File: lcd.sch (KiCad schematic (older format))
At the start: 13 parts, among them J10 FH26W-33S-0.3SHW, J7 AFA07-S10FCC-00, U8 AP3019A

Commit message: cleaned up libs
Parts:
- U8: symbol otter:AP3019A -> OtterCastAmp-rescue:AP3019A-otter
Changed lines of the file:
@@
 LEDK
 $Comp
-L otter:AP3019A U8
+L OtterCastAmp-rescue:AP3019A-otter U8
 U 1 1 60C69466
 P 3550 2350

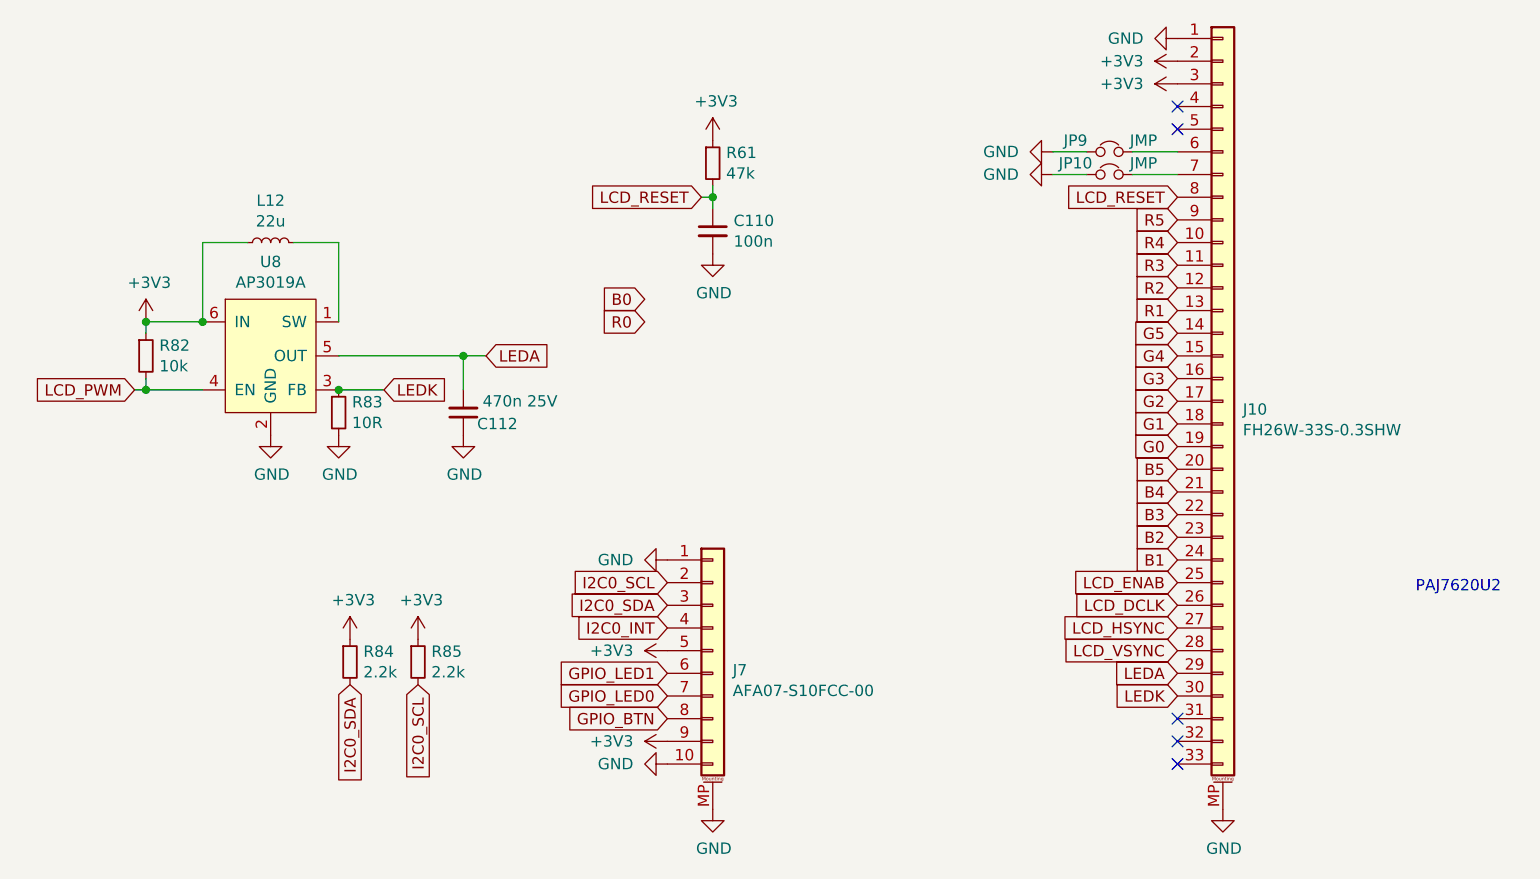
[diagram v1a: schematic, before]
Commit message: V1.2 production release
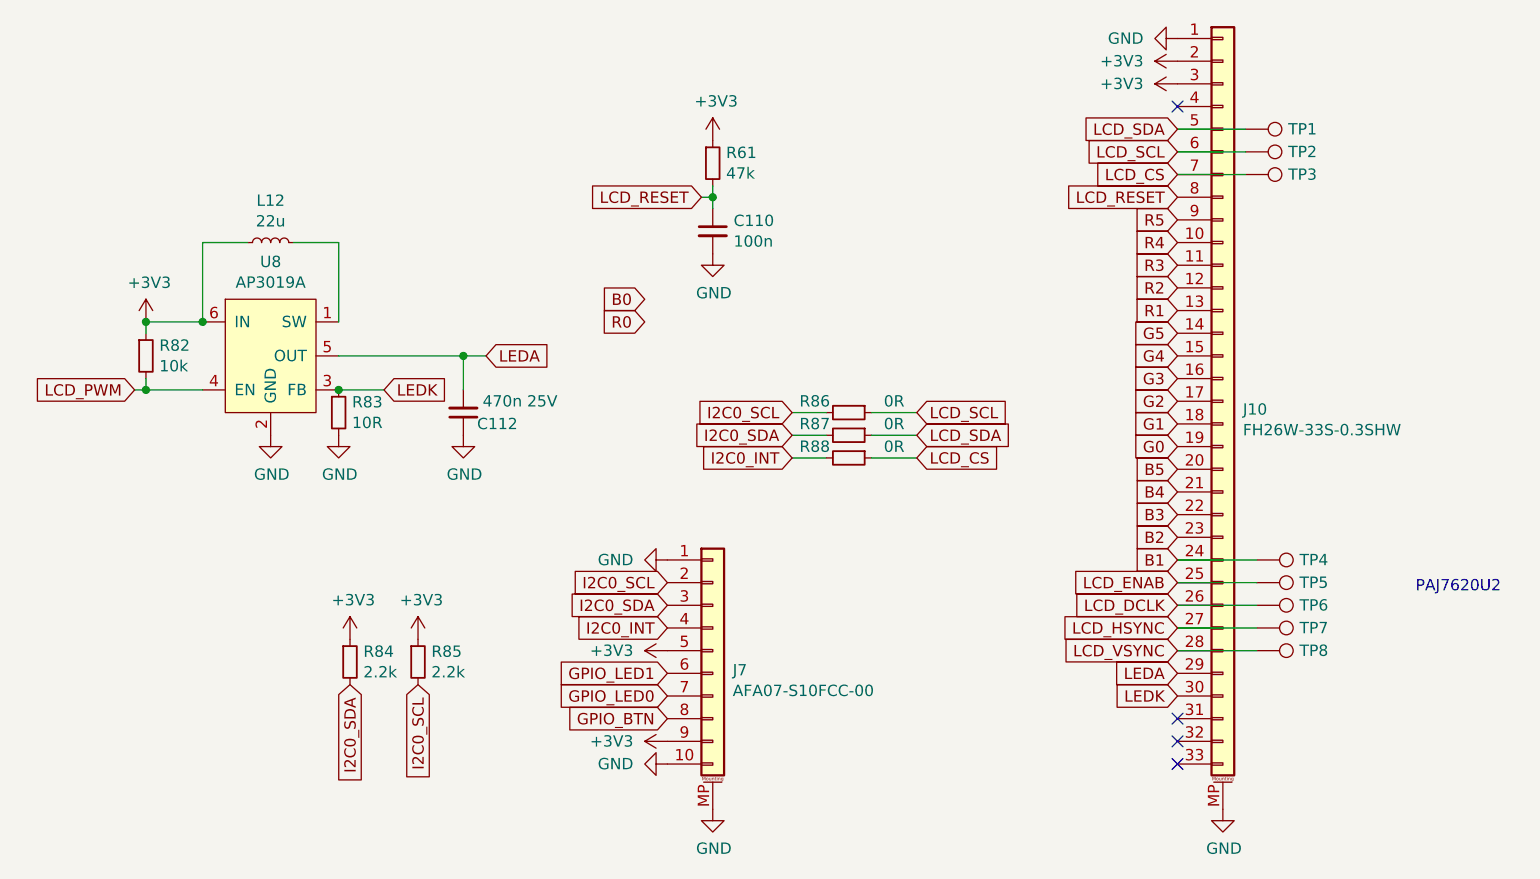
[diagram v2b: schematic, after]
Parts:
- removed JP10, JP9: JMP, Jumper:SolderJumper-2_P1.3mm_Bridged_Pad1.0x1.5mm, symbol Device:Jumper_NC_Small
- added R86, R87, R88: 0R, otter:R_0402, symbol Device:R_Small
- added TP1, TP2, TP3, TP4, TP5, TP6, TP7, TP8: TestPoint, TestPoint:TestPoint_Pad_1.0x1.0mm, symbol Connector:TestPoint
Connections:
- net B1: now also TP4.1
- net I2C0_INT: now also R88.2
- net I2C0_SCL: now also R86.2
- net I2C0_SDA: now also R87.2
- net LCD_DCLK: now also TP6.1
- net LCD_ENAB: now also TP5.1
- net LCD_HSYNC: now also TP7.1
- net LCD_VSYNC: now also TP8.1
- net LCD_SCL: now reaches J10.6 (Pin_6)
- net LCD_SCL: now also R86.1, TP2.1
- net LCD_CS: now reaches J10.7 (Pin_7)
- net LCD_CS: now also R88.1, TP3.1
- net LCD_SDA: now reaches J10.5 (Pin_5)
- net LCD_SDA: now also R87.1, TP1.1
- no-connect marks 5 -> 4
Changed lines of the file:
@@
 $EndComp
 NoConn ~ 7550 1250
-$Comp
-L Device:Jumper_NC_Small JP9
-U 1 1 60C3AE8C
-P 7250 1450
-F 0 "JP9" H 7100 1500 50  0000 C CNN
-F 1 "JMP" H 7400 1500 50  0000 C CNN
-F 2 "Jumper:SolderJumper-2_P1.3mm_Bridged_Pad1.0x1.5mm" H 7250 1450 50  0001 C CNN
-F 3 "~" H 7250 1450 50  0001 C CNN
-	1    7250 1450
-	1    0    0    -1
-$EndComp
-Wire Wire Line
-	7350 1550 7550 1550
-Wire Wire Line
-	7550 1450 7350 1450
-NoConn ~ 7550 1350
-$Comp
-L otter:GND #PWR0236
-U 1 1 60C3E844
-P 7000 1450
-F 0 "#PWR0236" H 7000 1200 50  0001 C CNN
-F 1 "GND" V 7000 1300 50  0000 R CNN
-F 2 "" H 7000 1450 60  0000 C CNN
-F 3 "" H 7000 1450 60  0000 C CNN
-	1    7000 1450
-	0    1    1    0
-$EndComp
-$Comp
-L otter:GND #PWR0237
-U 1 1 60C3EB01
-P 7000 1550
-F 0 "#PWR0237" H 7000 1300 50  0001 C CNN
-F 1 "GND" V 7000 1400 50  0000 R CNN
-F 2 "" H 7000 1550 60  0000 C CNN
-F 3 "" H 7000 1550 60  0000 C CNN
-	1    7000 1550
-	0    1    1    0
-$EndComp
-Wire Wire Line
-	7000 1550 7150 1550
-Wire Wire Line
-	7150 1450 7000 1450
-$Comp
-L Device:Jumper_NC_Small JP10
-U 1 1 60C3C276
-P 7250 1550
-F 0 "JP10" H 7100 1600 50  0000 C CNN
-F 1 "JMP" H 7400 1600 50  0000 C CNN
-F 2 "Jumper:SolderJumper-2_P1.3mm_Bridged_Pad1.0x1.5mm" H 7250 1550 50  0001 C CNN
-F 3 "~" H 7250 1550 50  0001 C CNN
-	1    7250 1550
-	1    0    0    -1
-$EndComp
 Text GLabel 7550 1650 0    50   Input ~ 0
 LCD_RESET
@@
 	0    -1   1    0
 $EndComp
+Text GLabel 7550 1350 0    50   Input ~ 0
+LCD_SDA
+Text GLabel 7550 1450 0    50   Input ~ 0
+LCD_SCL
+Text GLabel 7550 1550 0    50   Input ~ 0
+LCD_CS
+Text GLabel 5850 2600 0    50   Input ~ 0
+I2C0_SCL
+Text GLabel 5850 2700 0    50   Input ~ 0
+I2C0_SDA
+Text GLabel 5850 2800 0    50   Input ~ 0
+I2C0_INT
+$Comp
+L Device:R_Small R?
+U 1 1 6076BFC5
+P 6100 2600
+AR Path="/6076BFC5" Ref="R?"  Part="1"
+AR Path="/6145FE90/6076BFC5" Ref="R86"  Part="1"
+F 0 "R86" V 6050 2450 50  0000 C CNN
+F 1 "0R" V 6050 2800 50  0000 C CNN
+F 2 "otter:R_0402" H 6100 2600 50  0001 C CNN
+F 3 "~" H 6100 2600 50  0001 C CNN
+	1    6100 2600
+	0    1    1    0
+$EndComp
+$Comp
+L Device:R_Small R?
+U 1 1 6076C28C
+P 6100 2700
+AR Path="/6076C28C" Ref="R?"  Part="1"
+AR Path="/6145FE90/6076C28C" Ref="R87"  Part="1"
+F 0 "R87" V 6050 2550 50  0000 C CNN
+F 1 "0R" V 6050 2900 50  0000 C CNN
+F 2 "otter:R_0402" H 6100 2700 50  0001 C CNN
+F 3 "~" H 6100 2700 50  0001 C CNN
+	1    6100 2700
+	0    1    1    0
+$EndComp
+$Comp
+L Device:R_Small R?
+U 1 1 6076C4B4
+P 6100 2800
+AR Path="/6076C4B4" Ref="R?"  Part="1"
+AR Path="/6145FE90/6076C4B4" Ref="R88"  Part="1"
+F 0 "R88" V 6050 2650 50  0000 C CNN
+F 1 "0R" V 6050 3000 50  0000 C CNN
+F 2 "otter:R_0402" H 6100 2800 50  0001 C CNN
+F 3 "~" H 6100 2800 50  0001 C CNN
+	1    6100 2800
+	0    1    1    0
+$EndComp
+Text GLabel 6400 2700 2    50   Input ~ 0
+LCD_SDA
+Text GLabel 6400 2600 2    50   Input ~ 0
+LCD_SCL
+Text GLabel 6400 2800 2    50   Input ~ 0
+LCD_CS
+Wire Wire Line
+	6400 2600 6200 2600
+Wire Wire Line
+	6200 2700 6400 2700
+Wire Wire Line
+	6400 2800 6200 2800
+Wire Wire Line
+	6000 2800 5850 2800
+Wire Wire Line
+	5850 2700 6000 2700
+Wire Wire Line
+	6000 2600 5850 2600
+$Comp
+L Connector:TestPoint TP8
+U 1 1 6077A974
+P 7900 3650
+F 0 "TP8" V 7900 3838 50  0000 L CNN
+F 1 "TestPoint" V 7945 3838 50  0001 L CNN
+F 2 "TestPoint:TestPoint_Pad_1.0x1.0mm" H 8100 3650 50  0001 C CNN
+F 3 "~" H 8100 3650 50  0001 C CNN
+	1    7900 3650
+	0    1    1    0
+$EndComp
+$Comp
+L Connector:TestPoint TP7
+U 1 1 6077E3F5
+P 7900 3550
+F 0 "TP7" V 7900 3738 50  0000 L CNN
+F 1 "TestPoint" V 7945 3738 50  0001 L CNN
+F 2 "TestPoint:TestPoint_Pad_1.0x1.0mm" H 8100 3550 50  0001 C CNN
+F 3 "~" H 8100 3550 50  0001 C CNN
+	1    7900 3550
+	0    1    1    0
+$EndComp
+$Comp
+L Connector:TestPoint TP6
+U 1 1 6077E582
+P 7900 3450
+F 0 "TP6" V 7900 3638 50  0000 L CNN
+F 1 "TestPoint" V 7945 3638 50  0001 L CNN
+F 2 "TestPoint:TestPoint_Pad_1.0x1.0mm" H 8100 3450 50  0001 C CNN
+F 3 "~" H 8100 3450 50  0001 C CNN
+	1    7900 3450
+	0    1    1    0
+$EndComp
+$Comp
+L Connector:TestPoint TP5
+U 1 1 6077E815
+P 7900 3350
+F 0 "TP5" V 7900 3538 50  0000 L CNN
+F 1 "TestPoint" V 7945 3538 50  0001 L CNN
+F 2 "TestPoint:TestPoint_Pad_1.0x1.0mm" H 8100 3350 50  0001 C CNN
+F 3 "~" H 8100 3350 50  0001 C CNN
+	1    7900 3350
+	0    1    1    0
+$EndComp
+$Comp
+L Connector:TestPoint TP4
+U 1 1 6077EF76
+P 7900 3250
+F 0 "TP4" V 7900 3438 50  0000 L CNN
+F 1 "TestPoint" V 7945 3438 50  0001 L CNN
+F 2 "TestPoint:TestPoint_Pad_1.0x1.0mm" H 8100 3250 50  0001 C CNN
+F 3 "~" H 8100 3250 50  0001 C CNN
+	1    7900 3250
+	0    1    1    0
+$EndComp
+Wire Wire Line
+	7900 3250 7550 3250
+Wire Wire Line
+	7550 3350 7900 3350
+Wire Wire Line
+	7900 3450 7550 3450
+Wire Wire Line
+	7550 3550 7900 3550
+Wire Wire Line
+	7900 3650 7550 3650
+$Comp
+L Connector:TestPoint TP3
+U 1 1 6078578F
+P 7850 1550
+F 0 "TP3" V 7850 1738 50  0000 L CNN
+F 1 "TestPoint" V 7895 1738 50  0001 L CNN
+F 2 "TestPoint:TestPoint_Pad_1.0x1.0mm" H 8050 1550 50  0001 C CNN
+F 3 "~" H 8050 1550 50  0001 C CNN
+	1    7850 1550
+	0    1    1    0
+$EndComp
+$Comp
+L Connector:TestPoint TP2
+U 1 1 60785795
+P 7850 1450
+F 0 "TP2" V 7850 1638 50  0000 L CNN
+F 1 "TestPoint" V 7895 1638 50  0001 L CNN
+F 2 "TestPoint:TestPoint_Pad_1.0x1.0mm" H 8050 1450 50  0001 C CNN
+F 3 "~" H 8050 1450 50  0001 C CNN
+	1    7850 1450
+	0    1    1    0
+$EndComp
+$Comp
+L Connector:TestPoint TP1
+U 1 1 6078579B
+P 7850 1350
+F 0 "TP1" V 7850 1538 50  0000 L CNN
+F 1 "TestPoint" V 7895 1538 50  0001 L CNN
+F 2 "TestPoint:TestPoint_Pad_1.0x1.0mm" H 8050 1350 50  0001 C CNN
+F 3 "~" H 8050 1350 50  0001 C CNN
+	1    7850 1350
+	0    1    1    0
+$EndComp
+Wire Wire Line
+	7850 1350 7550 1350
+Wire Wire Line
+	7550 1450 7850 1450
+Wire Wire Line
+	7850 1550 7550 1550
 $EndSCHEMATC
